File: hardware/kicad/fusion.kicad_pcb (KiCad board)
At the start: 2 copper layers, 33 x 59.9 mm, 36 parts, among them J1 BATTERY, J2 LSM6DSOX, J3 PICKIT, J4 HC-05, J5 FLEX, J7 FTDI, SW1 BUTTON, SW2 POWER, SW3 UART, U1 MCP1603, U2 PIC16F690

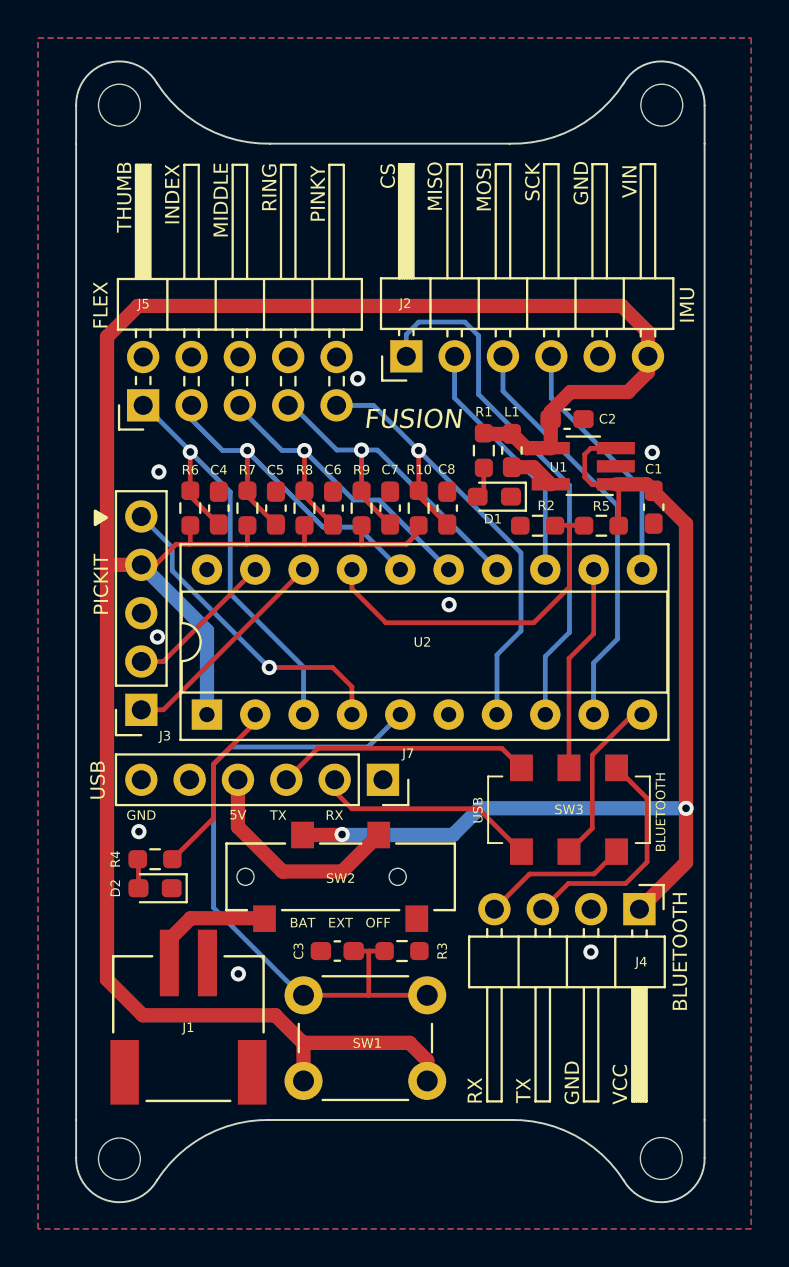
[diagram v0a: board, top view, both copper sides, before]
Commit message: Implement Chung's feedback for PCB
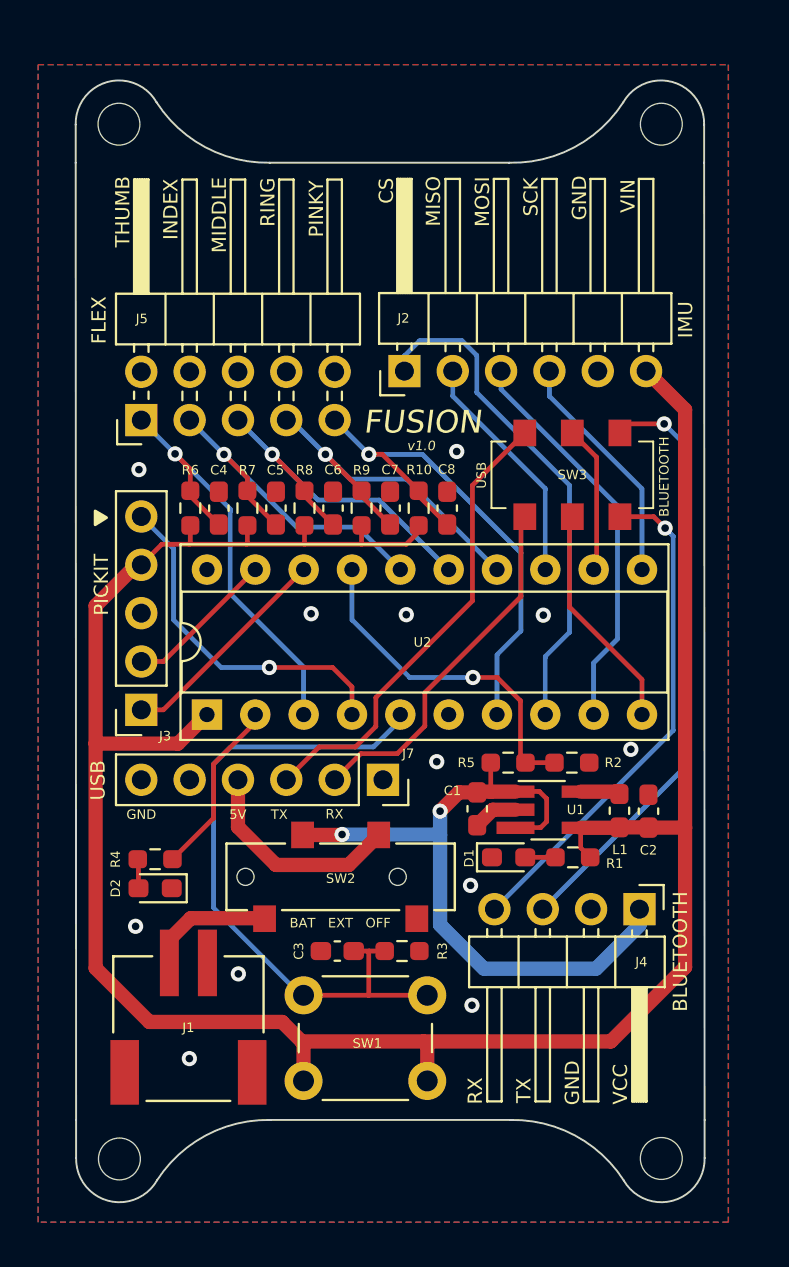
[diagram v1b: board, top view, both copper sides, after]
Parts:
- moved R1 21.9 mm to (163.1, 105.5), turned to 0 degrees
- moved C2 21.0 mm to (167.1, 103.1), turned to 90 degrees
- moved L1 19.8 mm to (165.6, 103.0), turned to -90 degrees
- moved D1 19.0 mm to (159.7, 105.5), turned to 0 degrees
- moved C1 18.4 mm to (158.1, 103.0)
- moved U1 18.1 mm to (161.8, 103.0), turned to 0 degrees
- moved SW3 17.6 mm to (163.1, 85.4)
- moved R5 13.4 mm to (159.7, 100.5), turned to 0 degrees
- moved R2 12.6 mm to (163.1, 100.5), turned to 0 degrees
- moved REF** 1.00 mm to (139.3, 67.0)
- moved REF** 1.00 mm to (167.8, 67.0)
- moved J2 0.78 mm to (154.2, 80.0)
- moved J5 0.78 mm to (140.4, 82.5)
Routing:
- net BT_RX: track 7.67 -> 26.7 mm, vias 0 -> 1
- net BT_TX: track 12.1 -> 31.0 mm, vias 0 -> 1
- net VDC: track 53.3 -> 37.1 mm
- net USB_TX: track 13.5 -> 24.5 mm
- net USB_RX: track 11.1 -> 18.8 mm
- net RX: track 11.0 -> 7.55 mm
- net +3V3: track 129.3 -> 125.9 mm
- net TX: track 8.59 -> 11.8 mm
- net GNDREF: track 0.00 -> 2.35 mm, vias 8 -> 12
- net MCLR: track 17.0 -> 18.4 mm
- net CS: track 27.9 -> 26.7 mm
- net PINKY: track 26.2 -> 27.2 mm
- net SCK: track 13.2 -> 12.4 mm
- net MISO: track 13.2 -> 12.4 mm
- net MOSI: track 21.8 -> 21.1 mm
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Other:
- board size 33 x 59.9 mm -> 33 x 58.9 mm
- board text added: "v1.0"
